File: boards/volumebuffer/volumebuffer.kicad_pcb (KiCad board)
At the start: 2 copper layers, 63.8 x 36.1 mm, 35 parts, among them P1 CONN_01X07, P2 CONN_01X03, U1 TL074, U2 TL072

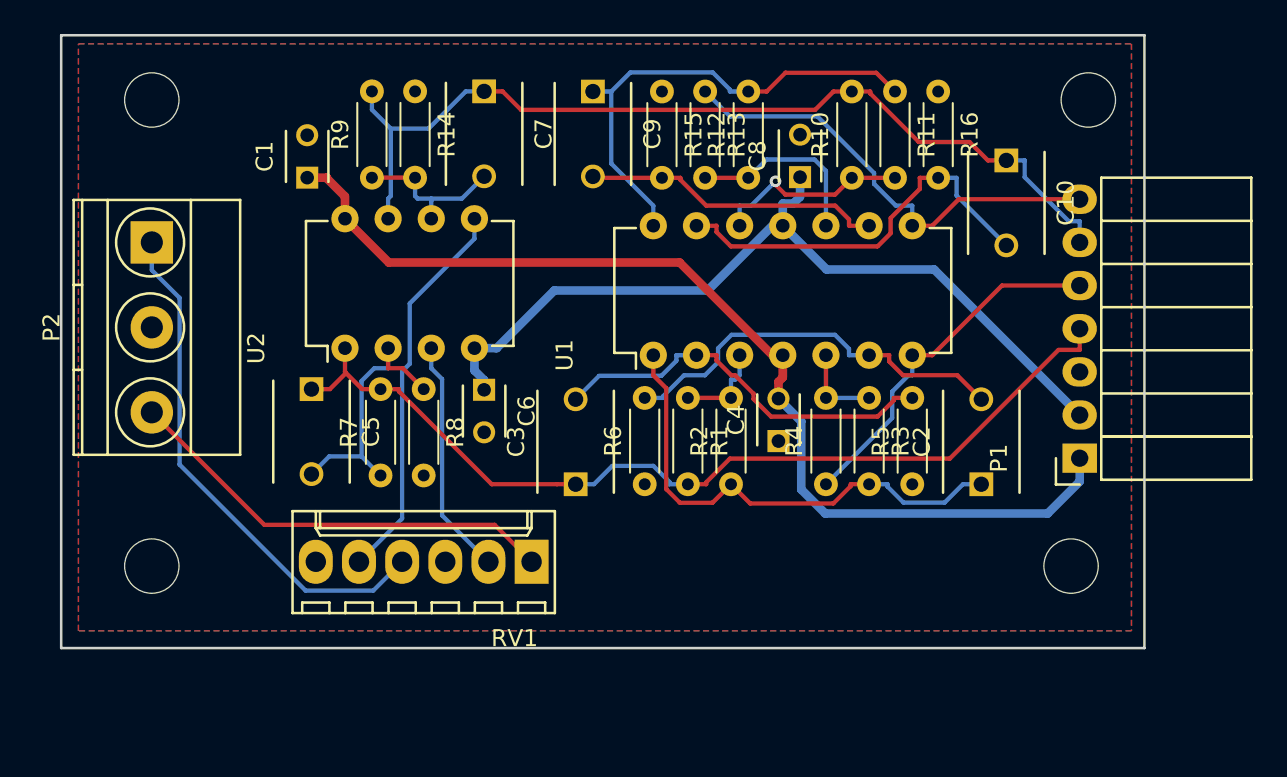
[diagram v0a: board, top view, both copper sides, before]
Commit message: more boards work
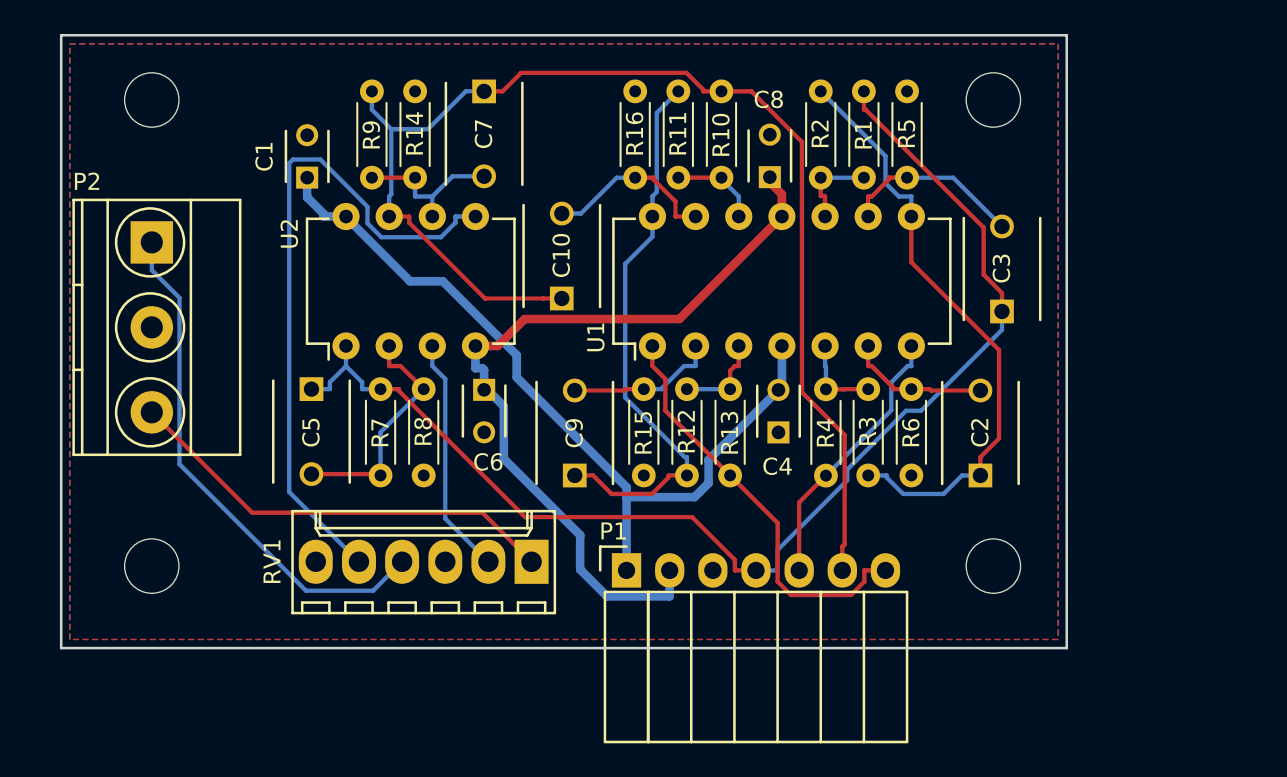
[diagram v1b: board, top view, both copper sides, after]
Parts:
- moved P1 27.5 mm to (61.7, 47.2), turned to 0 degrees
- moved C10 27.4 mm to (57.9, 31.2), turned to 90 degrees
- moved C3 27.1 mm to (83.8, 32.0)
- moved R2 23.7 mm to (73.2, 19.1), turned to 270 degrees
- moved R5 23.1 mm to (78.2, 19.1), turned to 270 degrees
- moved R13 22.6 mm to (67.8, 41.7), turned to 90 degrees
- moved C9 22.6 mm to (58.7, 41.7), turned to 90 degrees
- moved R15 22.6 mm to (62.7, 41.7), turned to 90 degrees
- moved R16 17.8 mm to (62.2, 19.1)
- moved R1 16.6 mm to (75.7, 24.1), turned to 90 degrees
- moved R6 15.7 mm to (78.5, 41.7)
- moved R12 13.0 mm to (65.3, 36.6), turned to 270 degrees
- moved R11 12.8 mm to (64.8, 19.1)
- moved R10 7.67 mm to (67.3, 24.1)
- moved mnt3 5.59 mm to (83.3, 19.6)
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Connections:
- U1 pad 1: Net-(C2-Pad1) -> /right_tweet
- U1 pad 10: Net-(R12-Pad1) -> Net-(R1-Pad1)
- U1 pad 2: Net-(C3-Pad2) -> Net-(C9-Pad2)
- U1 pad 3: Net-(R1-Pad1) -> Net-(R12-Pad1)
- U1 pad 8: /right_tweet -> Net-(C2-Pad1)
- U1 pad 9: Net-(C9-Pad2) -> Net-(C3-Pad2)
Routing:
- net /right_bass: track 55.4 -> 73.9 mm
- net /left_bass: track 55.4 -> 72.7 mm
- net Net-(RV1-Pad5): track 23.0 -> 39.4 mm
- net Net-(C2-Pad2): track 23.9 -> 8.45 mm
- net Net-(C10-Pad2): track 23.8 -> 10.3 mm
- net +15V: track 61.1 -> 47.8 mm
- net Net-(C3-Pad2): track 23.5 -> 10.8 mm
- net Net-(C9-Pad2): track 17.7 -> 8.93 mm
- net Net-(R10-Pad1): track 11.8 -> 5.25 mm, vias 1 -> 0
- net Net-(C2-Pad1): track 29.5 -> 35.4 mm
- net Net-(R12-Pad1): track 11.1 -> 5.43 mm
- net /left_tweet: track 21.4 -> 16.1 mm
- net Net-(C9-Pad1): track 28.6 -> 33.1 mm
- net /right_tweet: track 27.0 -> 24.6 mm
- net -15V: track 49.8 -> 47.4 mm
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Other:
- board size 63.8 x 36.1 mm -> 59.2 x 36.1 mm
